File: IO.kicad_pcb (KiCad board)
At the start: 2 copper layers, 68.6 x 66 mm, 10 parts

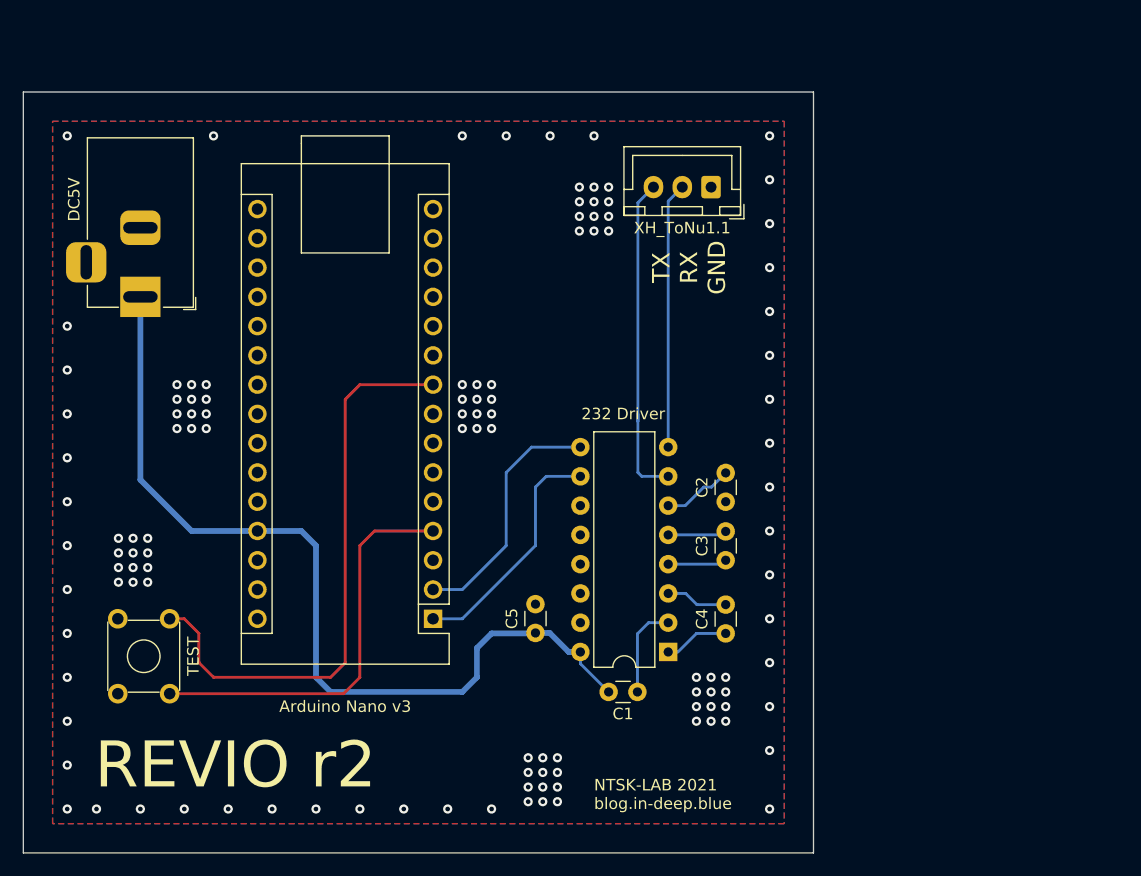
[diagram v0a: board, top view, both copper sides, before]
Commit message: 穴あけ前
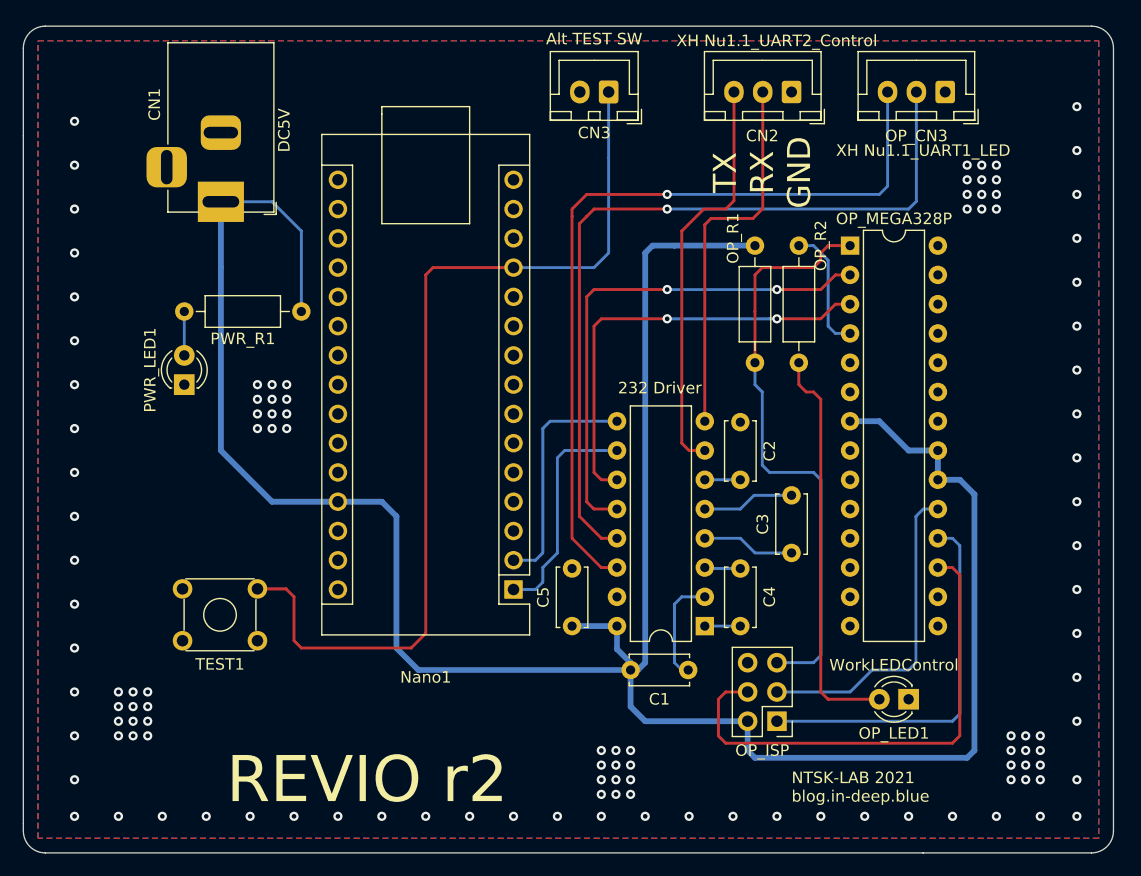
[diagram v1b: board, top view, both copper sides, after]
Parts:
- added CN3: Alt TEST SW, Connector_JST:JST_XH_B2B-XH-A_1x02_P2.50mm_Vertical, F.Cu at (114.3, 48.3)
- added OP_CN3: XH Nu1.1_UART1_LED, Connector_JST:JST_XH_B3B-XH-A_1x03_P2.50mm_Vertical, F.Cu at (143.5, 48.3)
- added OP_ISP: Conn_01x06, Connector_PinHeader_2.54mm:PinHeader_2x03_P2.54mm_Vertical, F.Cu at (128.9, 102.9)
- added OP_LED1: WorkLEDControl, LED_THT:LED_D3.0mm, F.Cu at (140.3, 101.0)
- added OP_MEGA328P: ATmega328P-PU, Package_DIP:DIP-28_W7.62mm, F.Cu at (135.3, 61.6)
- added OP_R1: 10k, Resistor_THT:R_Axial_DIN0207_L6.3mm_D2.5mm_P10.16mm_Horizontal, F.Cu at (127.0, 71.8)
- added OP_R2: 1k, Resistor_THT:R_Axial_DIN0207_L6.3mm_D2.5mm_P10.16mm_Horizontal, F.Cu at (130.8, 71.8)
- added PWR_LED1: PwrOK, LED_THT:LED_D3.0mm, F.Cu at (77.5, 73.7)
- added PWR_R1: 1k, Resistor_THT:R_Axial_DIN0207_L6.3mm_D2.5mm_P10.16mm_Horizontal, F.Cu at (87.6, 67.3)
- 232 Driver: value ADM232A -> MAX232
- C1, C2, C3, C4, C5: value C_Small -> 0.1u; footprint Capacitor_THT:C_Disc_D3.0mm_W1.6mm_P2.50mm -> Capacitor_THT:C_Disc_D5.0mm_W2.5mm_P5.00mm
- CN1: renamed from DC5V; value Conn_Coaxial_Power -> DC5V
- CN2: renamed from XH_ToNu1.1; value Conn_01x03 -> XH Nu1.1_UART2_Control
- Nano1: renamed from Arduino Nano v3
- moved CN2 10.8 mm to (130.2, 48.3)
- moved CN1 10.8 mm to (80.6, 57.8)
- moved TEST1 7.85 mm to (83.8, 95.9), turned to 180 degrees
- moved Nano1 7.43 mm to (106.0, 91.4)
- moved C3 5.75 mm to (130.2, 88.3)
- moved 232 Driver 3.89 mm to (122.6, 94.6)
- moved C5 3.23 mm to (111.1, 94.6)
- moved C1 2.69 mm to (116.2, 98.4)
- moved C2 2.29 mm to (125.7, 81.9)
- moved C4 1.42 mm to (125.7, 94.6)
- renumbered TEST to TEST1
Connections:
- 232 Driver pad 11: (no net) -> Net-(OP_U2-Pad3)
- 232 Driver pad 12: (no net) -> Net-(OP_U2-Pad2)
- 232 Driver pad 13: (no net) -> Net-(OP_CN3-Pad2)
- 232 Driver pad 14: (no net) -> Net-(OP_CN3-Pad3)
- 232 Driver pad 6: Net-(ADM232-Pad6) -> Net-(C2-Pad1)
- C2 pad 1: GND -> Net-(C2-Pad1)
- C2 pad 2: Net-(ADM232-Pad6) -> GND
- Nano1 pad 12: (no net) -> Net-(CN3-Pad1)
- Nano1 pad 4: Net-(Nano1-Pad4) -> GND
- Nano1 pad 9: Net-(Nano1-Pad9) -> (no net)
- TEST1 pad 1: Net-(Nano1-Pad9) -> (no net)
- TEST1 pad 2: Net-(Nano1-Pad4) -> GND
- TEST1 pad 3: (no net) -> Net-(CN3-Pad1)
- TEST1 pad 4: (no net) -> GND
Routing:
- net +5V: track 77.2 -> 216.0 mm
- net Net-(CN3-Pad1): track 0.00 -> 81.2 mm
- net Net-(OP_CN3-Pad3): track 0.00 -> 69.9 mm, vias 0 -> 1
- net Net-(OP_CN3-Pad2): track 0.00 -> 69.0 mm, vias 0 -> 1
- net Net-(OP_ISP1-Pad5): track 0.00 -> 51.4 mm
- net Net-(Nano1-Pad9): track 50.4 -> 0.00 mm
- net Net-(OP_U2-Pad2): track 0.00 -> 44.3 mm, vias 0 -> 2
- net Net-(OP_ISP1-Pad4): track 0.00 -> 43.6 mm
- net Net-(OP_U2-Pad3): track 0.00 -> 38.0 mm, vias 0 -> 2
- net Net-(Nano1-Pad4): track 35.4 -> 0.00 mm
- net Net-(OP_LED1-Pad2): track 0.00 -> 35.1 mm
- net Net-(OP_ISP1-Pad1): track 0.00 -> 32.9 mm
- net Net-(OP_ISP1-Pad3): track 0.00 -> 28.0 mm
- net Net-(OP_R2-Pad2): track 0.00 -> 10.9 mm
- net Net-(CN2-Pad2): track 23.1 -> 32.8 mm
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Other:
- board size 68.6 x 66 mm -> 94.6 x 71.8 mm

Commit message: 穴あけ後
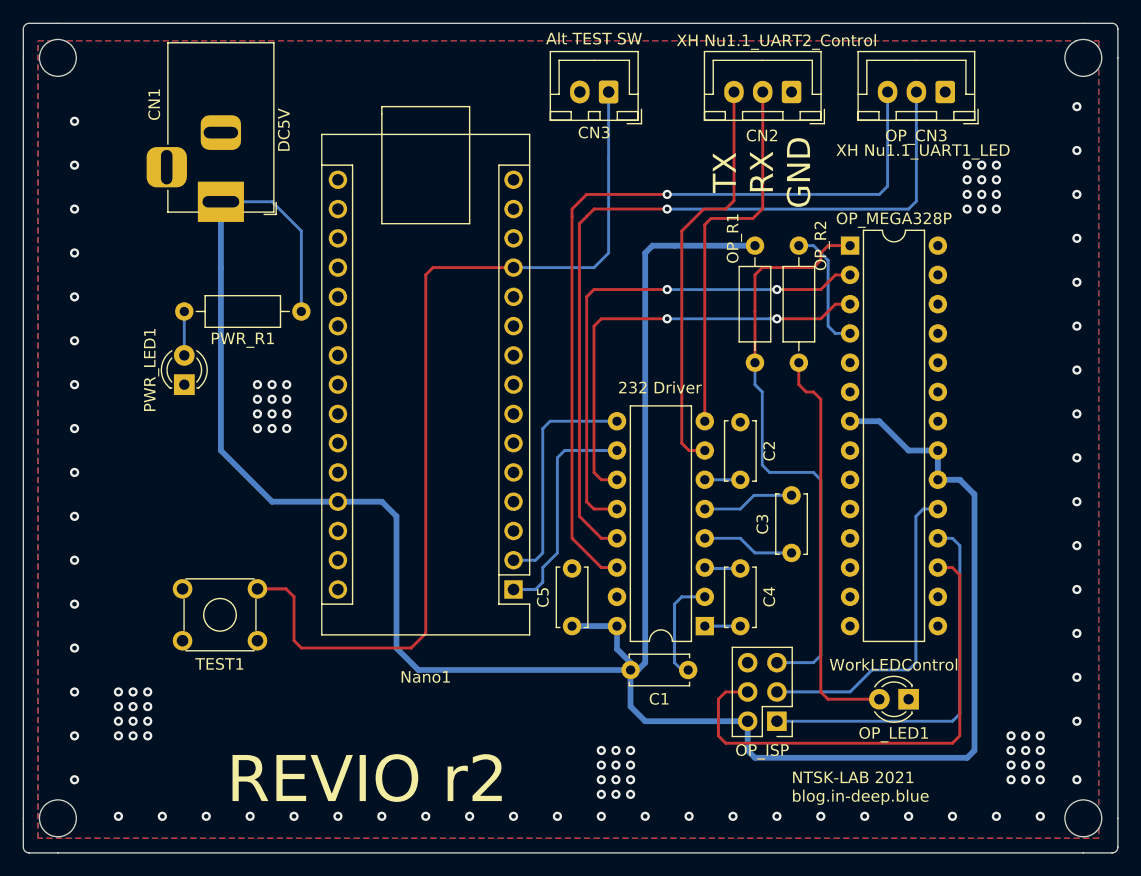
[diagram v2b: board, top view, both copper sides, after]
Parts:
- added REF**: MountingHole_3.2mm_M3, MountingHole:MountingHole_3.2mm_M3, F.Cu at (155.5, 45.3)
- added REF**: MountingHole_3.2mm_M3, MountingHole:MountingHole_3.2mm_M3, F.Cu at (155.5, 111.3)
- added REF**: MountingHole_3.2mm_M3, MountingHole:MountingHole_3.2mm_M3, F.Cu at (66.5, 111.3)
- added REF**: MountingHole_3.2mm_M3, MountingHole:MountingHole_3.2mm_M3, F.Cu at (66.5, 45.3)
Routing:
- net GND: vias 113 -> 114
- net (no net): vias 3 -> 0
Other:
- board size 94.6 x 71.8 mm -> 95 x 72 mm

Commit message: Revert "穴あけ後"
This reverts commit 9a31620a24121a6f974f63edfe8fbebed2765f06.
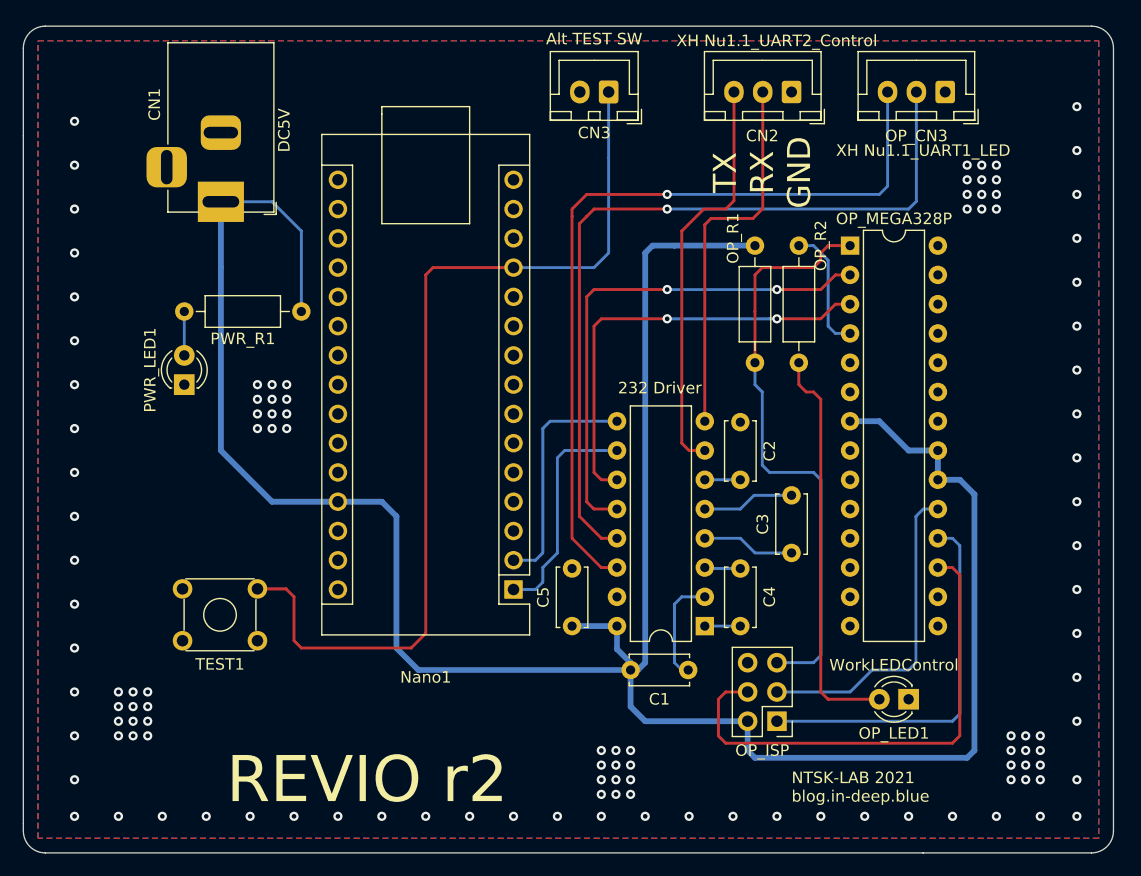
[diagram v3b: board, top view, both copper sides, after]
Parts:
- removed REF** (x4): MountingHole_3.2mm_M3, MountingHole:MountingHole_3.2mm_M3
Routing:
- net GND: vias 114 -> 113
- net (no net): vias 0 -> 3
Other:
- board size 95 x 72 mm -> 94.6 x 71.8 mm
